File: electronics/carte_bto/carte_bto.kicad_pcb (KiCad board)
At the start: 2 copper layers, 160 x 100 mm, 192 parts, among them J1 DIN41612_02x32_AB, J2 Conn_01x01, J3 Conn_01x01, J4 Conn_01x01, J5 Conn_01x01, J6 Conn_01x01, Q1 MMBT2222A, Q10 MMBT2222A, Q11 MMBT2222A, Q12 MMBT2222A, Q13 MMBT2222A, Q14 MMBT2222A, Q15 MMBT2222A, Q16 MMBT2222A, Q17 MMBT2222A, Q18 MMBT2222A, Q2 MMBT2222A, Q3 MMBT2222A, Q4 MMBT2222A, Q5 MMBT2222A, Q6 MMBT2222A, Q7 MMBT2222A, Q8 MMBT2222A, Q9 MMBT2222A, U1 74AHC541, U2 LTC1859IG_PBF, U3 LT6654AIS6-2.5_TRPBF, U4 74AHC541, U5 L78L05_SOT89

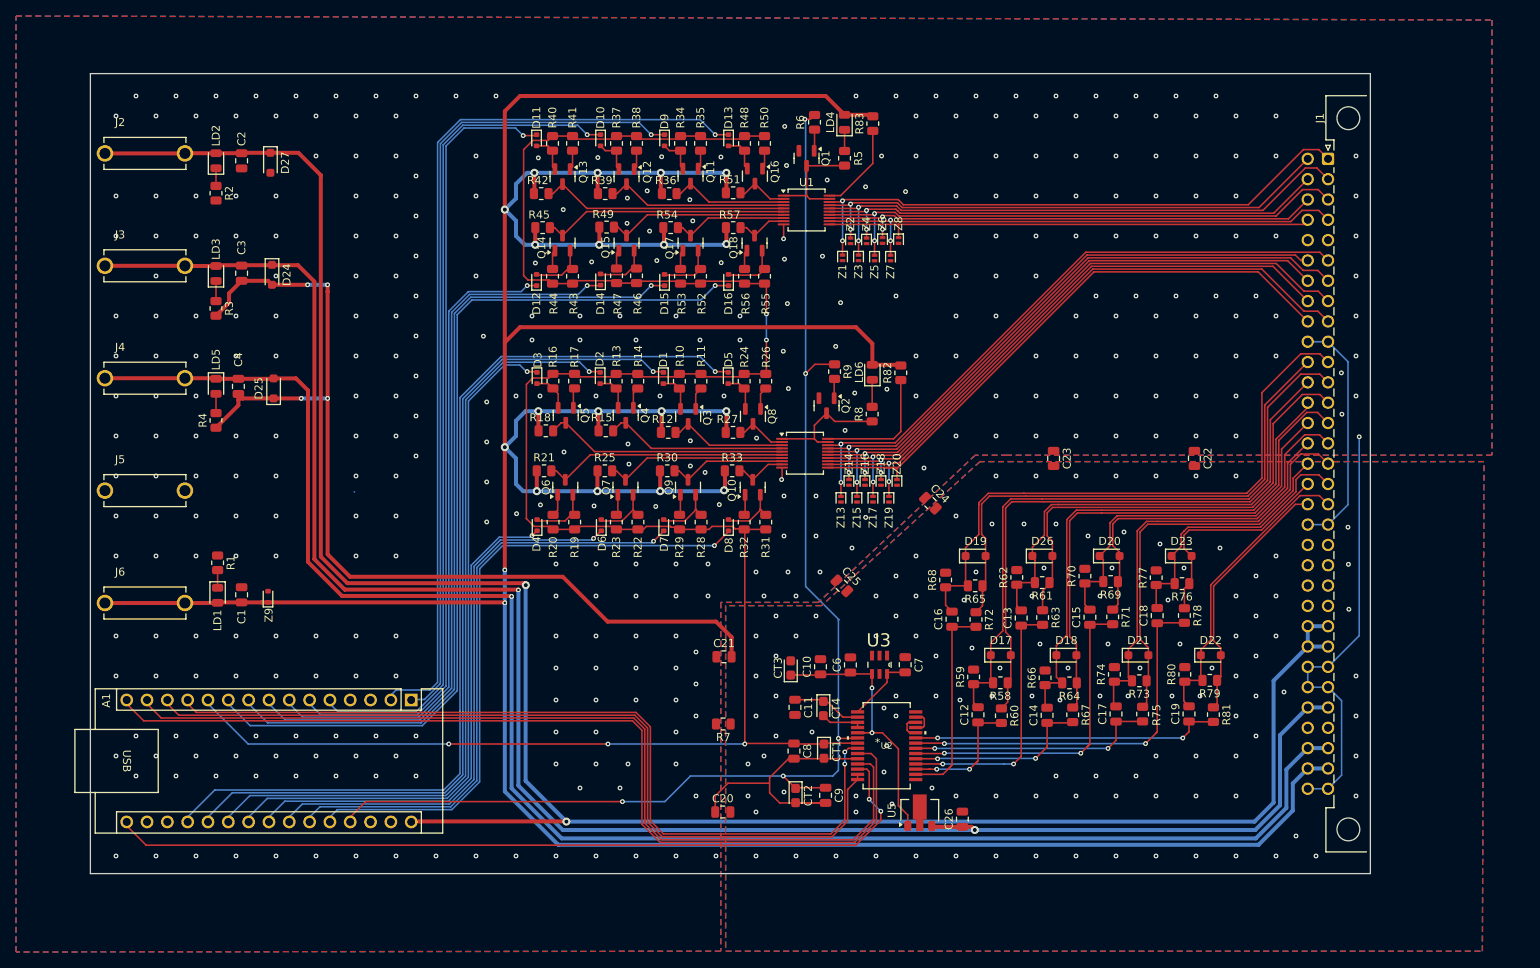
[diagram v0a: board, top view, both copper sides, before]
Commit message: BTO: Changed footprints to handsoldering verions, redid PCB routing
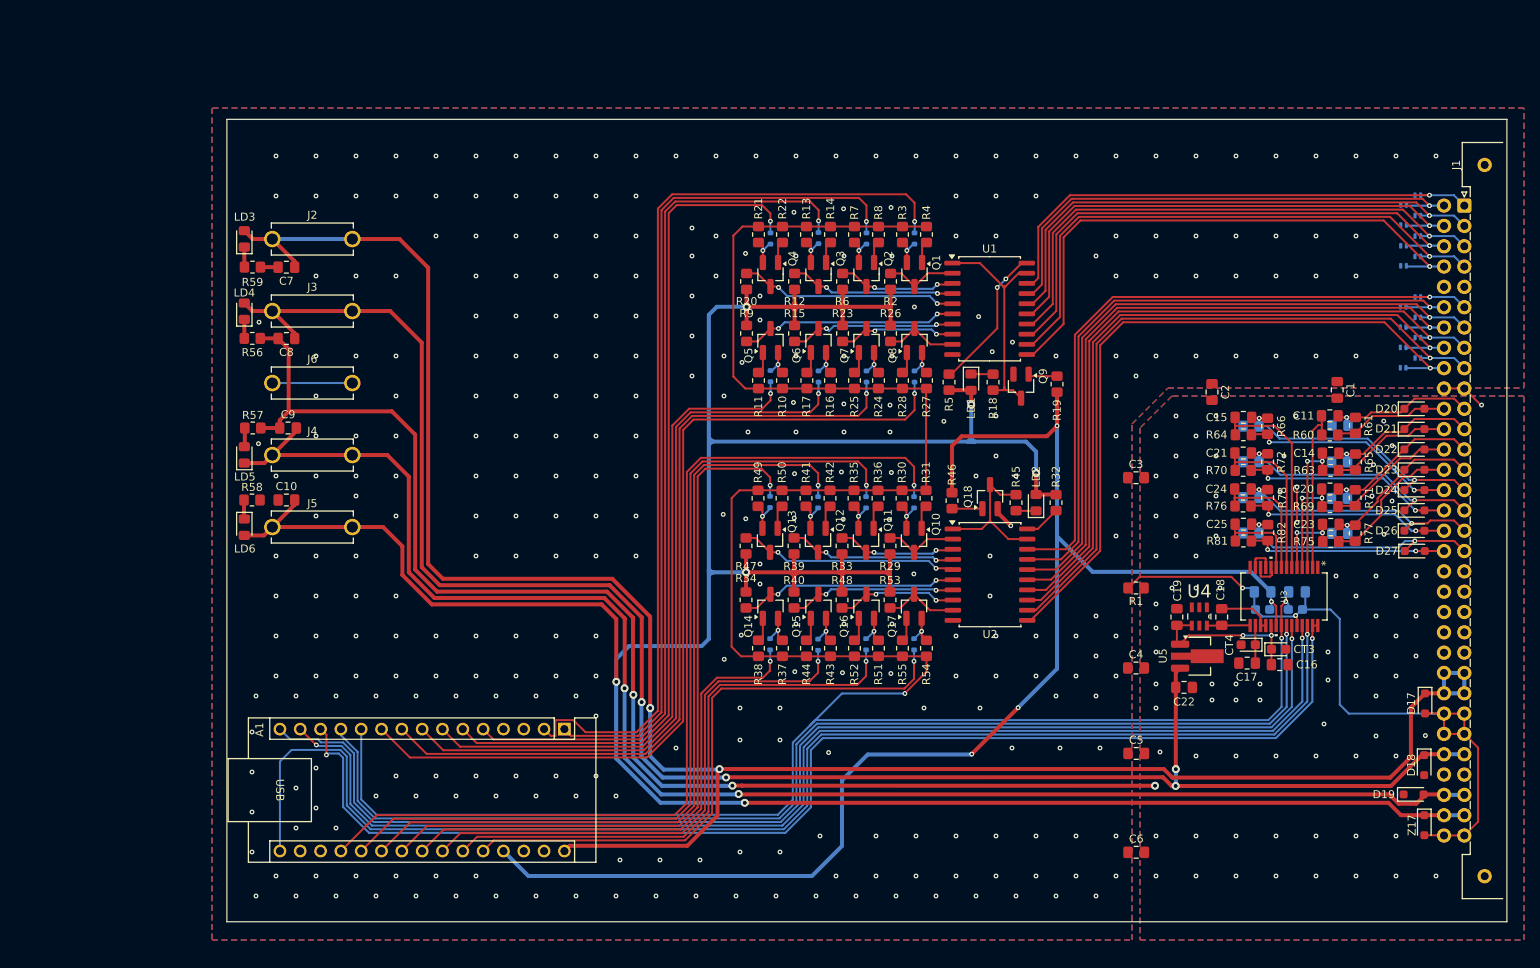
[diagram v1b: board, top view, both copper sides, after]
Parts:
- removed C26: 100nF, Capacitor_SMD:C_0805_2012Metric
- removed Z18, Z19, Z20: PESD5V0L1UL, Diode_SMD:D_SOD-882
- added C5: C_Small, Capacitor_SMD:C_0805_2012Metric_Pad1.18x1.45mm_HandSolder, F.Cu at (187.5, 124.7)
- added Z10: PESD5V0L1UL, PCM_Diode_SMD_Handsoldering_AKL:D_SOD-882_DFN1006-2_TVS, B.Cu at (220.9, 68.9)
- added Z11: PESD5V0L1UL, PCM_Diode_SMD_Handsoldering_AKL:D_SOD-882_DFN1006-2_TVS, B.Cu at (222.7, 70.2)
- added Z12: PESD5V0L1UL, PCM_Diode_SMD_Handsoldering_AKL:D_SOD-882_DFN1006-2_TVS, B.Cu at (220.9, 71.4)
- C1, C2, C3, C4: value 4.7µF -> C_Small; footprint Capacitor_SMD:C_0805_2012Metric -> Capacitor_SMD:C_0805_2012Metric_Pad1.18x1.45mm_HandSolder
- C10, C7, C8, C9: value 100nF -> 4.7µF; footprint Capacitor_SMD:C_0805_2012Metric -> Capacitor_SMD:C_0805_2012Metric_Pad1.18x1.45mm_HandSolder
- C11: value 100nF -> 1.5nF; footprint Capacitor_SMD:C_0805_2012Metric -> Capacitor_SMD:C_0805_2012Metric_Pad1.18x1.45mm_HandSolder
- C12, C13: value 1.5nF -> 100nF; footprint Capacitor_SMD:C_0805_2012Metric -> Capacitor_SMD:C_0805_2012Metric_Pad1.18x1.45mm_HandSolder; moved to B.Cu
- C14, C15: footprint Capacitor_SMD:C_0805_2012Metric -> Capacitor_SMD:C_0805_2012Metric_Pad1.18x1.45mm_HandSolder
- C16, C17, C18: value 1.5nF -> 100nF; footprint Capacitor_SMD:C_0805_2012Metric -> Capacitor_SMD:C_0805_2012Metric_Pad1.18x1.45mm_HandSolder
- C19: value 1.5nF -> 10µF; footprint Capacitor_SMD:C_0805_2012Metric -> Capacitor_SMD:C_0805_2012Metric_Pad1.18x1.45mm_HandSolder
- C20, C21, C23, C24, C25: value C_Small -> 1.5nF; footprint Capacitor_SMD:C_0805_2012Metric -> Capacitor_SMD:C_0805_2012Metric_Pad1.18x1.45mm_HandSolder
- C22: value C_Small -> 100nF; footprint Capacitor_SMD:C_0805_2012Metric -> Capacitor_SMD:C_0805_2012Metric_Pad1.18x1.45mm_HandSolder
- C6: value 10µF -> C_Small; footprint Capacitor_SMD:C_0805_2012Metric -> Capacitor_SMD:C_0805_2012Metric_Pad1.18x1.45mm_HandSolder
- CT1, CT2: moved to B.Cu
- D1, D10, D11, D12, D13, D14, D15, D16, D2, D3, D4, D5, D6, D7, D8, D9: footprint Diode_SMD:D_SOD-523 -> PCM_Diode_SMD_Handsoldering_AKL:D_SOD-523; moved to B.Cu
- D17: value SMAJ12CA -> SMAJ12A
- D18, D19: value SMAJ12CA -> SMAJ15A
- D20: value SMAJ12CA -> PESD12VL1BA
- D24, D25: value SMAJ15A -> SMAJ12CA
- D27: value SMAJ12A -> SMAJ12CA
- J1: footprint Connector_DIN:DIN41612_B_2x32_Male_Horizontal_THT -> connecteur_europe:DIN41612_B_2x32_Male_Horizontal_THT
- LD1, LD2: value LED_Small -> LED; footprint LED_SMD:LED_0805_2012Metric -> LED_SMD:LED_0805_2012Metric_Pad1.15x1.40mm_HandSolder
- LD3, LD5: footprint LED_SMD:LED_0805_2012Metric -> LED_SMD:LED_0805_2012Metric_Pad1.15x1.40mm_HandSolder
- LD4, LD6: value LED -> LED_Small; footprint LED_SMD:LED_0805_2012Metric -> LED_SMD:LED_0805_2012Metric_Pad1.15x1.40mm_HandSolder
- Q1, Q10, Q11, Q12, Q13, Q14, Q15, Q16, Q17, Q18, Q2, Q3, Q4, Q5, Q6, Q7, Q8, Q9: footprint Package_TO_SOT_SMD:SOT-23 -> Package_TO_SOT_SMD:SOT-23_Handsoldering
- R1, R5: value 3.3k -> 0; footprint Resistor_SMD:R_0805_2012Metric -> Resistor_SMD:R_0805_2012Metric_Pad1.20x1.40mm_HandSolder
- R10, R11, R12, R13, R16, R17, R21, R22, R23, R24, R27, R30, R33, R34, R37, R38, R39, R40, R43, R44, R48, R49, R50, R51, R54, R60, R61, R63, R65, R75, R81: footprint Resistor_SMD:R_0805_2012Metric -> Resistor_SMD:R_0805_2012Metric_Pad1.20x1.40mm_HandSolder
- R14, R20, R26, R29, R35, R41, R47, R53, R6, R9: value 22k -> 10k; footprint Resistor_SMD:R_0805_2012Metric -> Resistor_SMD:R_0805_2012Metric_Pad1.20x1.40mm_HandSolder
- R15, R19, R25, R28, R31, R36, R42, R46, R52, R55: value 10k -> 22k; footprint Resistor_SMD:R_0805_2012Metric -> Resistor_SMD:R_0805_2012Metric_Pad1.20x1.40mm_HandSolder
- R18, R45: value 10k -> 3.3k; footprint Resistor_SMD:R_0805_2012Metric -> Resistor_SMD:R_0805_2012Metric_Pad1.20x1.40mm_HandSolder
- R2, R3: value 5.1k -> 10k; footprint Resistor_SMD:R_0805_2012Metric -> Resistor_SMD:R_0805_2012Metric_Pad1.20x1.40mm_HandSolder
- R32: value 22k -> 0; footprint Resistor_SMD:R_0805_2012Metric -> Resistor_SMD:R_0805_2012Metric_Pad1.20x1.40mm_HandSolder
- R4: value 5.1k -> 22k; footprint Resistor_SMD:R_0805_2012Metric -> Resistor_SMD:R_0805_2012Metric_Pad1.20x1.40mm_HandSolder
- R56: value 22k -> 5.1k; footprint Resistor_SMD:R_0805_2012Metric -> Resistor_SMD:R_0805_2012Metric_Pad1.20x1.40mm_HandSolder
- R57: value 10k -> 5.1k; footprint Resistor_SMD:R_0805_2012Metric -> Resistor_SMD:R_0805_2012Metric_Pad1.20x1.40mm_HandSolder
- R58: value 1M -> 3.3k; footprint Resistor_SMD:R_0805_2012Metric -> Resistor_SMD:R_0805_2012Metric_Pad1.20x1.40mm_HandSolder
- R59: value 100 -> 5.1k; footprint Resistor_SMD:R_0805_2012Metric -> Resistor_SMD:R_0805_2012Metric_Pad1.20x1.40mm_HandSolder
- R62, R68, R74, R80: footprint Resistor_SMD:R_0805_2012Metric -> Resistor_SMD:R_0805_2012Metric_Pad1.20x1.40mm_HandSolder; moved to B.Cu
- R64, R69, R76: value 1M -> 10k; footprint Resistor_SMD:R_0805_2012Metric -> Resistor_SMD:R_0805_2012Metric_Pad1.20x1.40mm_HandSolder
- R66, R77: value 100 -> 1M; footprint Resistor_SMD:R_0805_2012Metric -> Resistor_SMD:R_0805_2012Metric_Pad1.20x1.40mm_HandSolder
- R67: value 10k -> 100; footprint Resistor_SMD:R_0805_2012Metric -> Resistor_SMD:R_0805_2012Metric_Pad1.20x1.40mm_HandSolder; moved to B.Cu
- R7: value 0 -> 10k; footprint Resistor_SMD:R_0805_2012Metric -> Resistor_SMD:R_0805_2012Metric_Pad1.20x1.40mm_HandSolder
- R70: value 100 -> 10k; footprint Resistor_SMD:R_0805_2012Metric -> Resistor_SMD:R_0805_2012Metric_Pad1.20x1.40mm_HandSolder
- R71, R72, R78: value 10k -> 1M; footprint Resistor_SMD:R_0805_2012Metric -> Resistor_SMD:R_0805_2012Metric_Pad1.20x1.40mm_HandSolder
- R73, R79: value 1M -> 100; footprint Resistor_SMD:R_0805_2012Metric -> Resistor_SMD:R_0805_2012Metric_Pad1.20x1.40mm_HandSolder; moved to B.Cu
- R8: value 3.3k -> 22k; footprint Resistor_SMD:R_0805_2012Metric -> Resistor_SMD:R_0805_2012Metric_Pad1.20x1.40mm_HandSolder
- R82: value 0 -> 1M; footprint Resistor_SMD:R_0805_2012Metric -> Resistor_SMD:R_0805_2012Metric_Pad1.20x1.40mm_HandSolder
- R83: value 0 -> 100; footprint Resistor_SMD:R_0805_2012Metric -> Resistor_SMD:R_0805_2012Metric_Pad1.20x1.40mm_HandSolder; moved to B.Cu
- U1: footprint Package_SO:TSSOP-20_4.4x5mm_P0.4mm -> Package_SO:SOIC-20W_7.5x12.8mm_P1.27mm
- U2: value LTC1859IG_PBF -> 74AHC541; footprint imported_components:SSOP-28_G -> Package_SO:SOIC-20W_7.5x12.8mm_P1.27mm
- U3: value LT6654AIS6-2.5_TRPBF -> LTC1859IG_PBF; footprint imported_components:SOT95P280X100-6N -> imported_components:SSOP-28_G
- U4: value 74AHC541 -> LT6654AIS6-2.5_TRPBF; footprint Package_SO:TSSOP-20_4.4x5mm_P0.4mm -> imported_components:SOT95P280X100-6N
- U5: footprint Package_TO_SOT_SMD:SOT-89-3 -> Package_TO_SOT_SMD:SOT-89-3_Handsoldering
- Z1, Z13, Z14, Z15, Z16, Z2, Z3, Z4, Z5, Z6, Z7, Z8: footprint Diode_SMD:D_SOD-882 -> PCM_Diode_SMD_Handsoldering_AKL:D_SOD-882_DFN1006-2_TVS; moved to B.Cu
- Z17: value PESD5V0L1UL -> PESD5V0L1UA; footprint Diode_SMD:D_SOD-882 -> Diode_SMD:D_SOD-323_HandSoldering
- Z9: footprint Diode_SMD:D_SOD-523 -> PCM_Diode_SMD_Handsoldering_AKL:D_SOD-882_DFN1006-2_TVS; moved to B.Cu
- moved D27 151.1 mm to (222.3, 99.4), turned to 0 degrees
- moved Z9 148.5 mm to (222.7, 67.6), turned to 180 degrees
- moved D24 145.3 mm to (222.3, 91.8), turned to 0 degrees
- moved D25 143.4 mm to (222.3, 94.3), turned to 0 degrees
- moved C1 139.3 mm to (212.7, 79.2), turned to -90 degrees
- moved C2 124.7 mm to (197.0, 79.5)
- moved C4 117.6 mm to (187.5, 114.0), turned to 0 degrees
- moved R1 114.8 mm to (187.5, 104.0), turned to 180 degrees
- moved C3 114.7 mm to (187.5, 90.2), turned to 0 degrees
- moved LD2 111.1 mm to (175.0, 93.3)
- moved R59 103.7 mm to (77.1, 63.9), turned to 0 degrees
- moved LD1 97.9 mm to (166.9, 78.3)
- moved R58 96.3 mm to (77.0, 93.0)
- moved C7 91.9 mm to (81.3, 63.9), turned to 180 degrees
- moved R4 91.8 mm to (161.3, 59.8), turned to -90 degrees
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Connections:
- net /d0 renamed /Bus donnée/OUT0
- net /d1 renamed /Bus donnée/OUT1
- net /d2 renamed /Bus donnée/OUT2
- net /d3 renamed /Bus donnée/OUT3
- net /d4 renamed /Bus donnée/OUT4
- net /d5 renamed /Bus donnée/OUT5
- net /d6 renamed /Bus donnée/OUT6
- net /d7 renamed /Bus donnée/OUT7
- A1 pad 12: /adc_busy -> /ADC 16 bits 8 voies/~{BUSY}
- A1 pad 13: /SPI.cs -> /ADC 16 bits 8 voies/SPI_CS
- A1 pad 14: /SPI.copi -> /ADC 16 bits 8 voies/SPI_COPI
- A1 pad 15: /SPI.cipo -> /ADC 16 bits 8 voies/SPI_CIPO
- A1 pad 16: /SPI.sck -> /ADC 16 bits 8 voies/SPI_SCK
- C1 pad 1: +5V -> GND2
- C1 pad 2: GND2 -> GND1
- C10 pad 1: +5VA -> +5V
- C10 pad 2: GND1 -> GND2
- C11 pad 1: Net-(U2-REFCOMP) -> /ADC 16 bits 8 voies/ch0
- C11 pad 2: GND1 -> /ADC 16 bits 8 voies/COM0_IN
- C12 pad 1: /Protections 8voies analogiques/CH1_OUT -> /ioref
- C12 pad 2: /acom1 -> GND2
- C13 pad 1: /Protections 8voies analogiques/CH2_OUT -> +5VARD
- C13 pad 2: /acom2 -> GND2
- C14 pad 1: /Protections 8voies analogiques/CH3_OUT -> /ADC 16 bits 8 voies/ch1
- C14 pad 2: /acom3 -> /ADC 16 bits 8 voies/COM1_IN
- C15 pad 1: /Protections 8voies analogiques/CH4_OUT -> /ADC 16 bits 8 voies/ch4
- C15 pad 2: /acom4 -> /ADC 16 bits 8 voies/COM4_IN
- C16 pad 1: /Protections 8voies analogiques/CH0_OUT -> +5VA
- C16 pad 2: /acom0 -> GND1
- C17 pad 1: /Protections 8voies analogiques/CH5_OUT -> Net-(U3-REFCOMP)
- C17 pad 2: /acom5 -> GND1
- C18 pad 1: /Protections 8voies analogiques/CH6_OUT -> Net-(U3-VREF)
- C18 pad 2: /acom6 -> GND1
- C19 pad 1: /Protections 8voies analogiques/CH7_OUT -> +5VA
- C19 pad 2: /acom7 -> GND1
- C2 pad 1: +12VP -> GND2
- C2 pad 2: GND2 -> GND1
- C20 pad 1: GND2 -> /ADC 16 bits 8 voies/ch2
- C20 pad 2: GND1 -> /ADC 16 bits 8 voies/COM2_IN
- C21 pad 1: GND2 -> /ADC 16 bits 8 voies/ch5
- C21 pad 2: GND1 -> /ADC 16 bits 8 voies/COM5_IN
- C22 pad 1: GND2 -> +15V
- C23 pad 1: GND2 -> /ADC 16 bits 8 voies/ch3
- C23 pad 2: GND1 -> /ADC 16 bits 8 voies/COM3_IN
- C24 pad 1: GND2 -> /ADC 16 bits 8 voies/ch6
- C24 pad 2: GND1 -> /ADC 16 bits 8 voies/COM6_IN
- C25 pad 1: GND2 -> /ADC 16 bits 8 voies/ch7
- C25 pad 2: GND1 -> /ADC 16 bits 8 voies/COM7_IN
- C3 pad 1: +15V -> GND2
- C4 pad 1: GND1 -> GND2
- C4 pad 2: -15V -> GND1
- C6 pad 1: +5VA -> GND2
- C7 pad 1: Net-(U2-VREF) -> +12VP
- C7 pad 2: GND1 -> GND2
- C8 pad 1: /ioref -> +15V
- C8 pad 2: GND2 -> GND1
- C9 pad 1: +5VARD -> GND1
- C9 pad 2: GND2 -> -15V
- CT4 pad 1: Net-(U2-REFCOMP) -> Net-(U3-REFCOMP)
- D1 pad 1: /addr1 -> /data0
- D10 pad 1: /data2 -> /addr1
- D11 pad 1: /data3 -> /addr2
- D12 pad 1: /data4 -> /addr3
- D13 pad 1: /data0 -> /addr4
- D14 pad 1: /data5 -> /addr5
- D15 pad 1: /data6 -> /addr6
- D16 pad 1: /data7 -> /addr7
- D17 pad 1: /acom1 -> +12VP
- D17 pad 2: /ach1 -> GND2
- D18 pad 1: /acom3 -> +15V
- D18 pad 2: /ach3 -> GND1
- D19 pad 1: /acom0 -> GND1
- D19 pad 2: /ach0 -> -15V
- D2 pad 1: /addr2 -> /data1
- D20 pad 1: /acom4 -> /ADC 16 bits 8 voies/COM0_IN
- D20 pad 2: /ach4 -> /ADC 16 bits 8 voies/CH0_IN
- D21 pad 1: /acom5 -> /ADC 16 bits 8 voies/COM1_IN
- D21 pad 2: /ach5 -> /ADC 16 bits 8 voies/CH1_IN
- D22 pad 1: /acom7 -> /ADC 16 bits 8 voies/COM2_IN
- D22 pad 2: /ach7 -> /ADC 16 bits 8 voies/CH2_IN
- D23 pad 1: /acom6 -> /ADC 16 bits 8 voies/COM3_IN
- D23 pad 2: /ach6 -> /ADC 16 bits 8 voies/CH3_IN
- D24 pad 1: +15V -> /ADC 16 bits 8 voies/COM4_IN
- D24 pad 2: GND1 -> /ADC 16 bits 8 voies/CH4_IN
- D25 pad 1: GND1 -> /ADC 16 bits 8 voies/COM5_IN
- D25 pad 2: -15V -> /ADC 16 bits 8 voies/CH5_IN
- D26 pad 1: /acom2 -> /ADC 16 bits 8 voies/COM6_IN
- D26 pad 2: /ach2 -> /ADC 16 bits 8 voies/CH6_IN
- D27 pad 1: +12VP -> /ADC 16 bits 8 voies/COM7_IN
- D27 pad 2: GND2 -> /ADC 16 bits 8 voies/CH7_IN
- D3 pad 1: /addr3 -> /data2
- D4 pad 1: /addr4 -> /data3
- D5 pad 1: /addr0 -> /data4
- D6 pad 1: /addr5 -> /data5
- D7 pad 1: /addr6 -> /data6
- D8 pad 1: /addr7 -> /data7
- D9 pad 1: /data1 -> /addr0
- J1 pad a11: /acom0 -> /ADC 16 bits 8 voies/COM0_IN
- J1 pad a12: /acom1 -> /ADC 16 bits 8 voies/COM1_IN
- J1 pad a13: /acom2 -> /ADC 16 bits 8 voies/COM2_IN
- J1 pad a14: /acom3 -> /ADC 16 bits 8 voies/COM3_IN
- J1 pad a15: /acom4 -> /ADC 16 bits 8 voies/COM4_IN
- J1 pad a16: /acom5 -> /ADC 16 bits 8 voies/COM5_IN
- J1 pad a17: /acom6 -> /ADC 16 bits 8 voies/COM6_IN
- J1 pad a18: /acom7 -> /ADC 16 bits 8 voies/COM7_IN
- J1 pad a6: /a0 -> /Bus d’adresse/OUT0
- J1 pad a7: /a2 -> /Bus d’adresse/OUT2
- J1 pad a8: /a4 -> /Bus d’adresse/OUT4
- J1 pad a9: /a6 -> /Bus d’adresse/OUT6
- J1 pad b11: /ach0 -> /ADC 16 bits 8 voies/CH0_IN
- J1 pad b12: /ach1 -> /ADC 16 bits 8 voies/CH1_IN
- J1 pad b13: /ach2 -> /ADC 16 bits 8 voies/CH2_IN
- J1 pad b14: /ach3 -> /ADC 16 bits 8 voies/CH3_IN
- J1 pad b15: /ach4 -> /ADC 16 bits 8 voies/CH4_IN
- J1 pad b16: /ach5 -> /ADC 16 bits 8 voies/CH5_IN
- J1 pad b17: /ach6 -> /ADC 16 bits 8 voies/CH6_IN
- J1 pad b18: /ach7 -> /ADC 16 bits 8 voies/CH7_IN
- J1 pad b6: /a1 -> /Bus d’adresse/OUT1
- J1 pad b7: /a3 -> /Bus d’adresse/OUT3
- J1 pad b8: /a5 -> /Bus d’adresse/OUT5
- J1 pad b9: /a7 -> /Bus d’adresse/OUT7
- J5 pad 1_1: GND2 -> +5V
- J5 pad 1_2: GND2 -> +5V
- J6 pad 1_1: +5V -> GND2
- J6 pad 1_2: +5V -> GND2
- LD2 pad 2: +12VP -> +5V
- LD3 pad 2: +15V -> +12VP
- LD4 pad 2: +5V -> +15V
- Q1 pad 2: GND2 -> Net-(D1-A)
- Q1 pad 3: Net-(Q1-C) -> /Bus donnée/bit0
- Q10 pad 2: Net-(D8-A) -> Net-(D9-A)
- Q10 pad 3: /Adaptateur 3v3 - 5v 8voies (1)/OUT7 -> /Bus d’adresse/bit0
- Q11 pad 2: Net-(D9-A) -> Net-(D10-A)
- Q11 pad 3: /Adaptateur 3v3 - 5v 8voies (2)/OUT1 -> /Bus d’adresse/bit1
- Q12 pad 2: Net-(D10-A) -> Net-(D11-A)
- Q12 pad 3: /Adaptateur 3v3 - 5v 8voies (2)/OUT2 -> /Bus d’adresse/bit2
- Q13 pad 2: Net-(D11-A) -> Net-(D12-A)
- Q13 pad 3: /Adaptateur 3v3 - 5v 8voies (2)/OUT3 -> /Bus d’adresse/bit3
- Q14 pad 2: Net-(D12-A) -> Net-(D13-A)
- Q14 pad 3: /Adaptateur 3v3 - 5v 8voies (2)/OUT4 -> /Bus d’adresse/bit4
- Q15 pad 3: /Adaptateur 3v3 - 5v 8voies (2)/OUT5 -> /Bus d’adresse/bit5
- Q16 pad 2: Net-(D13-A) -> Net-(D15-A)
- Q16 pad 3: /Adaptateur 3v3 - 5v 8voies (2)/OUT0 -> /Bus d’adresse/bit6
- Q17 pad 2: Net-(D15-A) -> Net-(D16-A)
- Q17 pad 3: /Adaptateur 3v3 - 5v 8voies (2)/OUT6 -> /Bus d’adresse/bit7
- Q18 pad 2: Net-(D16-A) -> GND2
- Q18 pad 3: /Adaptateur 3v3 - 5v 8voies (2)/OUT7 -> Net-(Q18-C)
- Q2 pad 2: GND2 -> Net-(D2-A)
- Q2 pad 3: Net-(Q2-C) -> /Bus donnée/bit1
- Q3 pad 2: Net-(D1-A) -> Net-(D3-A)
- Q3 pad 3: /Adaptateur 3v3 - 5v 8voies (1)/OUT1 -> /Bus donnée/bit2
- Q4 pad 2: Net-(D2-A) -> Net-(D4-A)
- Q4 pad 3: /Adaptateur 3v3 - 5v 8voies (1)/OUT2 -> /Bus donnée/bit3
- Q5 pad 2: Net-(D3-A) -> Net-(D5-A)
- Q5 pad 3: /Adaptateur 3v3 - 5v 8voies (1)/OUT3 -> /Bus donnée/bit4
- Q6 pad 2: Net-(D4-A) -> Net-(D6-A)
- Q6 pad 3: /Adaptateur 3v3 - 5v 8voies (1)/OUT4 -> /Bus donnée/bit5
- Q7 pad 2: Net-(D6-A) -> Net-(D7-A)
- Q7 pad 3: /Adaptateur 3v3 - 5v 8voies (1)/OUT5 -> /Bus donnée/bit6
- Q8 pad 2: Net-(D5-A) -> Net-(D8-A)
- Q8 pad 3: /Adaptateur 3v3 - 5v 8voies (1)/OUT0 -> /Bus donnée/bit7
- Q9 pad 2: Net-(D7-A) -> GND2
- Q9 pad 3: /Adaptateur 3v3 - 5v 8voies (1)/OUT6 -> Net-(Q9-C)
- R1 pad 1: GND2 -> GND1
- R1 pad 2: Net-(LD1-K) -> GND2
- R10 pad 2: Net-(D1-A) -> Net-(D5-A)
- R11 pad 2: Net-(Q3-B) -> Net-(Q5-B)
- R12 pad 2: /Adaptateur 3v3 - 5v 8voies (1)/OUT1 -> /Bus donnée/bit2
- R13 pad 2: Net-(D2-A) -> Net-(D3-A)
- R14 pad 2: Net-(Q4-B) -> Net-(Q3-B)
- R15 pad 2: /Adaptateur 3v3 - 5v 8voies (1)/OUT2 -> /Bus donnée/bit5
- R16 pad 2: Net-(D3-A) -> Net-(D6-A)
- R17 pad 2: Net-(Q5-B) -> Net-(Q6-B)
- R18 pad 1: +5V -> Net-(Q9-C)
- R18 pad 2: /Adaptateur 3v3 - 5v 8voies (1)/OUT3 -> Net-(LD1-K)
- R19 pad 1: /ioref -> +5VARD
- R19 pad 2: Net-(D4-A) -> Net-(Q9-B)
- R2 pad 1: Net-(LD2-K) -> +5V
- R2 pad 2: GND2 -> /Bus donnée/bit0
- R20 pad 1: /ioref -> +5V
- R20 pad 2: Net-(Q6-B) -> /Bus donnée/bit3
- R21 pad 1: +5V -> /ioref
- R21 pad 2: /Adaptateur 3v3 - 5v 8voies (1)/OUT4 -> Net-(D4-A)
- R22 pad 2: Net-(D6-A) -> Net-(Q4-B)
- R23 pad 1: /ioref -> +5V
- R23 pad 2: Net-(Q7-B) -> /Bus donnée/bit6
- R24 pad 2: Net-(D5-A) -> Net-(D7-A)
- R25 pad 1: +5V -> /ioref
- R25 pad 2: /Adaptateur 3v3 - 5v 8voies (1)/OUT5 -> Net-(Q7-B)
- R26 pad 1: /ioref -> +5V
- R26 pad 2: Net-(Q8-B) -> /Bus donnée/bit7
- R27 pad 1: +5V -> /ioref
- R27 pad 2: /Adaptateur 3v3 - 5v 8voies (1)/OUT0 -> Net-(D8-A)
- R28 pad 2: Net-(D7-A) -> Net-(Q8-B)
- R29 pad 1: /ioref -> +5V
- R29 pad 2: Net-(Q9-B) -> /Bus d’adresse/bit0
- R3 pad 1: Net-(LD3-K) -> /ioref
- R3 pad 2: GND1 -> Net-(D1-A)
- R30 pad 1: +5V -> /ioref
- R30 pad 2: /Adaptateur 3v3 - 5v 8voies (1)/OUT6 -> Net-(D9-A)
- R31 pad 2: Net-(D8-A) -> Net-(Q10-B)
- R32 pad 1: /ioref -> Net-(U2-VCC)
- R32 pad 2: Net-(Q10-B) -> +5V
- R33 pad 2: /Adaptateur 3v3 - 5v 8voies (1)/OUT7 -> /Bus d’adresse/bit1
- R34 pad 1: /ioref -> +5V
- R34 pad 2: Net-(D9-A) -> /Bus d’adresse/bit4
- R35 pad 2: Net-(Q11-B) -> Net-(D10-A)
- R36 pad 1: +5V -> /ioref
- R36 pad 2: /Adaptateur 3v3 - 5v 8voies (2)/OUT1 -> Net-(Q11-B)
- R37 pad 2: Net-(D10-A) -> Net-(D13-A)
- R38 pad 2: Net-(Q12-B) -> Net-(Q14-B)
- R39 pad 2: /Adaptateur 3v3 - 5v 8voies (2)/OUT2 -> /Bus d’adresse/bit2
- R4 pad 1: GND1 -> /ioref
- R4 pad 2: Net-(LD5-A) -> Net-(Q1-B)
- R40 pad 1: /ioref -> +5V
- R40 pad 2: Net-(D11-A) -> /Bus d’adresse/bit5
- R41 pad 2: Net-(Q13-B) -> Net-(D11-A)
- R42 pad 1: +5V -> /ioref
- R42 pad 2: /Adaptateur 3v3 - 5v 8voies (2)/OUT3 -> Net-(Q12-B)
- R43 pad 2: Net-(D12-A) -> Net-(D14-A)
- R44 pad 2: Net-(Q14-B) -> Net-(Q15-B)
- R45 pad 1: +5V -> Net-(Q18-C)
- R45 pad 2: /Adaptateur 3v3 - 5v 8voies (2)/OUT4 -> Net-(LD2-K)
- R46 pad 1: /ioref -> +5VARD
- R46 pad 2: Net-(D14-A) -> Net-(Q18-B)
- R47 pad 1: /ioref -> +5V
- R47 pad 2: Net-(Q15-B) -> /Bus d’adresse/bit3
- R48 pad 1: /ioref -> +5V
- R48 pad 2: Net-(D13-A) -> /Bus d’adresse/bit6
- R49 pad 1: +5V -> /ioref
- R49 pad 2: /Adaptateur 3v3 - 5v 8voies (2)/OUT5 -> Net-(D12-A)
- R5 pad 1: Net-(Q1-C) -> Net-(U1-VCC)
- R5 pad 2: Net-(LD4-K) -> +5V
- R50 pad 2: Net-(Q16-B) -> Net-(Q13-B)
- R51 pad 1: +5V -> /ioref
- R51 pad 2: /Adaptateur 3v3 - 5v 8voies (2)/OUT0 -> Net-(D15-A)
- R52 pad 2: Net-(D15-A) -> Net-(Q16-B)
- R53 pad 1: /ioref -> +5V
- R53 pad 2: Net-(Q17-B) -> /Bus d’adresse/bit7
- R54 pad 1: +5V -> /ioref
- R54 pad 2: /Adaptateur 3v3 - 5v 8voies (2)/OUT6 -> Net-(D16-A)
- R55 pad 2: Net-(D16-A) -> Net-(Q17-B)
- R56 pad 1: /ioref -> Net-(LD4-K)
- R56 pad 2: Net-(Q18-B) -> GND1
- R57 pad 1: +5V -> GND1
- R57 pad 2: /Adaptateur 3v3 - 5v 8voies (2)/OUT7 -> Net-(LD5-A)
- R58 pad 1: /ach1 -> GND2
- R58 pad 2: /acom1 -> Net-(LD6-K)
- R59 pad 1: /acom1 -> Net-(LD3-K)
- R59 pad 2: GND1 -> GND2
- R6 pad 1: +5VARD -> +5V
- R6 pad 2: Net-(Q1-B) -> /Bus donnée/bit1
- R60 pad 1: /ach1 -> /ADC 16 bits 8 voies/CH0_IN
- R60 pad 2: /Protections 8voies analogiques/CH1_OUT -> /ADC 16 bits 8 voies/ch0
- R61 pad 1: /ach2 -> /ADC 16 bits 8 voies/CH0_IN
- R61 pad 2: /acom2 -> /ADC 16 bits 8 voies/COM0_IN
- R62 pad 1: /acom2 -> /ADC 16 bits 8 voies/COM0_IN
- R63 pad 1: /ach2 -> /ADC 16 bits 8 voies/CH1_IN
- R63 pad 2: /Protections 8voies analogiques/CH2_OUT -> /ADC 16 bits 8 voies/ch1
- R64 pad 1: /ach3 -> /ADC 16 bits 8 voies/CH4_IN
- R64 pad 2: /acom3 -> /ADC 16 bits 8 voies/ch4
- R65 pad 1: /ach0 -> /ADC 16 bits 8 voies/CH1_IN
- R65 pad 2: /acom0 -> /ADC 16 bits 8 voies/COM1_IN
- R66 pad 1: /acom3 -> /ADC 16 bits 8 voies/CH4_IN
- R66 pad 2: GND1 -> /ADC 16 bits 8 voies/COM4_IN
- R67 pad 1: /ach3 -> /ADC 16 bits 8 voies/COM1_IN
- R67 pad 2: /Protections 8voies analogiques/CH3_OUT -> GND1
- R68 pad 1: /acom0 -> /ADC 16 bits 8 voies/COM4_IN
- R69 pad 1: /ach4 -> /ADC 16 bits 8 voies/CH2_IN
- R69 pad 2: /acom4 -> /ADC 16 bits 8 voies/ch2
- R7 pad 1: GND1 -> /ioref
- R7 pad 2: GND2 -> Net-(D2-A)
- R70 pad 1: /acom4 -> /ADC 16 bits 8 voies/CH5_IN
- R70 pad 2: GND1 -> /ADC 16 bits 8 voies/ch5
- R71 pad 1: /ach4 -> /ADC 16 bits 8 voies/CH2_IN
- R71 pad 2: /Protections 8voies analogiques/CH4_OUT -> /ADC 16 bits 8 voies/COM2_IN
- R72 pad 1: /ach0 -> /ADC 16 bits 8 voies/CH5_IN
- R72 pad 2: /Protections 8voies analogiques/CH0_OUT -> /ADC 16 bits 8 voies/COM5_IN
- R73 pad 1: /ach5 -> /ADC 16 bits 8 voies/COM2_IN
- R73 pad 2: /acom5 -> GND1
- R74 pad 1: /acom5 -> /ADC 16 bits 8 voies/COM5_IN
- R75 pad 1: /ach5 -> /ADC 16 bits 8 voies/CH3_IN
- R75 pad 2: /Protections 8voies analogiques/CH5_OUT -> /ADC 16 bits 8 voies/ch3
- R76 pad 1: /ach6 -> /ADC 16 bits 8 voies/CH6_IN
- R76 pad 2: /acom6 -> /ADC 16 bits 8 voies/ch6
- R77 pad 1: /acom6 -> /ADC 16 bits 8 voies/CH3_IN
- R77 pad 2: GND1 -> /ADC 16 bits 8 voies/COM3_IN
- R78 pad 1: /ach6 -> /ADC 16 bits 8 voies/CH6_IN
- R78 pad 2: /Protections 8voies analogiques/CH6_OUT -> /ADC 16 bits 8 voies/COM6_IN
- R79 pad 1: /ach7 -> /ADC 16 bits 8 voies/COM3_IN
- R79 pad 2: /acom7 -> GND1
- R8 pad 1: Net-(Q2-C) -> /ioref
- R8 pad 2: Net-(LD6-K) -> Net-(Q2-B)
- R80 pad 1: /acom7 -> /ADC 16 bits 8 voies/COM6_IN
- R81 pad 1: /ach7 -> /ADC 16 bits 8 voies/CH7_IN
- R81 pad 2: /Protections 8voies analogiques/CH7_OUT -> /ADC 16 bits 8 voies/ch7
- R82 pad 1: Net-(U4-VCC) -> /ADC 16 bits 8 voies/CH7_IN
- R82 pad 2: +5V -> /ADC 16 bits 8 voies/COM7_IN
- R83 pad 1: Net-(U1-VCC) -> /ADC 16 bits 8 voies/COM7_IN
- R83 pad 2: +5V -> GND1
- R9 pad 1: +5VARD -> +5V
- R9 pad 2: Net-(Q2-B) -> /Bus donnée/bit4
- U1 pad 1: Net-(Q1-C) -> Net-(Q9-C)
- U1 pad 19: Net-(Q1-C) -> Net-(Q9-C)
- U1 pad 2: /Adaptateur 3v3 - 5v 8voies (2)/OUT0 -> /Bus donnée/bit0
- U1 pad 3: /Adaptateur 3v3 - 5v 8voies (2)/OUT1 -> /Bus donnée/bit1
- U1 pad 4: /Adaptateur 3v3 - 5v 8voies (2)/OUT2 -> /Bus donnée/bit2
- U1 pad 5: /Adaptateur 3v3 - 5v 8voies (2)/OUT3 -> /Bus donnée/bit3
- U1 pad 6: /Adaptateur 3v3 - 5v 8voies (2)/OUT4 -> /Bus donnée/bit4
- U1 pad 7: /Adaptateur 3v3 - 5v 8voies (2)/OUT5 -> /Bus donnée/bit5
- U1 pad 8: /Adaptateur 3v3 - 5v 8voies (2)/OUT6 -> /Bus donnée/bit6
- U1 pad 9: /Adaptateur 3v3 - 5v 8voies (2)/OUT7 -> /Bus donnée/bit7
- U2 pad 1: GND1 -> Net-(Q18-C)
- U2 pad 10: Net-(U2-ADC+) -> GND2
- U2 pad 11: Net-(U2-ADC-) -> /Bus d’adresse/OUT7
- U2 pad 12: Net-(U2-ADC+) -> /Bus d’adresse/OUT6
- U2 pad 13: Net-(U2-ADC-) -> /Bus d’adresse/OUT5
- U2 pad 14: GND1 -> /Bus d’adresse/OUT4
- U2 pad 15: Net-(U2-VREF) -> /Bus d’adresse/OUT3
- U2 pad 16: Net-(U2-REFCOMP) -> /Bus d’adresse/OUT2
- U2 pad 17: GND1 -> /Bus d’adresse/OUT1
- U2 pad 18: GND1 -> /Bus d’adresse/OUT0
- U2 pad 19: +5VA -> Net-(Q18-C)
- U2 pad 2: /Protections 8voies analogiques/CH0_OUT -> /Bus d’adresse/bit0
- U2 pad 20: +5VARD -> Net-(U2-VCC)
- U2 pad 3: /Protections 8voies analogiques/CH1_OUT -> /Bus d’adresse/bit1
- U2 pad 4: /Protections 8voies analogiques/CH2_OUT -> /Bus d’adresse/bit2
- U2 pad 5: /Protections 8voies analogiques/CH3_OUT -> /Bus d’adresse/bit3
- U2 pad 6: /Protections 8voies analogiques/CH4_OUT -> /Bus d’adresse/bit4
- U2 pad 7: /Protections 8voies analogiques/CH5_OUT -> /Bus d’adresse/bit5
- U2 pad 8: /Protections 8voies analogiques/CH6_OUT -> /Bus d’adresse/bit6
- U2 pad 9: /Protections 8voies analogiques/CH7_OUT -> /Bus d’adresse/bit7
- U3 pad 2: GND1 -> /ADC 16 bits 8 voies/ch0
- U3 pad 3: unconnected-(U3-DNC-Pad3) -> /ADC 16 bits 8 voies/ch1
- U3 pad 4: +5VA -> /ADC 16 bits 8 voies/ch2
- U3 pad 5: unconnected-(U3-DNC_2-Pad5) -> /ADC 16 bits 8 voies/ch3
- U3 pad 6: Net-(U2-VREF) -> /ADC 16 bits 8 voies/ch4
- U4 pad 1: Net-(Q2-C) -> GND1
- U4 pad 2: /Adaptateur 3v3 - 5v 8voies (1)/OUT0 -> GND1
- U4 pad 3: /Adaptateur 3v3 - 5v 8voies (1)/OUT1 -> unconnected-(U4-DNC-Pad3)
- U4 pad 4: /Adaptateur 3v3 - 5v 8voies (1)/OUT2 -> +5VA
- U4 pad 5: /Adaptateur 3v3 - 5v 8voies (1)/OUT3 -> unconnected-(U4-DNC_2-Pad5)
- U4 pad 6: /Adaptateur 3v3 - 5v 8voies (1)/OUT4 -> Net-(U3-VREF)
- Z13 pad 1: /a0 -> /Bus d’adresse/OUT4
- Z14 pad 1: /a1 -> /Bus d’adresse/OUT5
- Z15 pad 1: /a2 -> /Bus d’adresse/OUT6
- Z16 pad 1: /a3 -> /Bus d’adresse/OUT7
- Z17 pad 1: /a4 -> +5V
- Z9 pad 1: +5V -> /Bus d’adresse/OUT0
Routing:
- net /ADC 16 bits 8 voies/SPI_SCK: track 0.00 -> 168.2 mm, vias 0 -> 1
- net /ADC 16 bits 8 voies/SPI_CS: track 0.00 -> 155.7 mm, vias 0 -> 2
- net /ADC 16 bits 8 voies/SPI_CIPO: track 0.00 -> 155.2 mm, vias 0 -> 1
- net /ADC 16 bits 8 voies/SPI_COPI: track 0.00 -> 154.0 mm, vias 0 -> 2
- net /ADC 16 bits 8 voies/~{BUSY}: track 0.00 -> 146.7 mm, vias 0 -> 1
- net /SPI.cipo: track 119.7 -> 0.00 mm
- net /SPI.copi: track 115.0 -> 0.00 mm
- net +5V: track 511.5 -> 400.2 mm, vias 20 -> 6
- net /adc_busy: track 107.2 -> 0.00 mm, vias 2 -> 0
- net /SPI.cs: track 106.4 -> 0.00 mm
- net /SPI.sck: track 105.2 -> 0.00 mm, vias 2 -> 0
- net /Bus d’adresse/OUT6: track 0.00 -> 88.4 mm, vias 0 -> 1
- net /Bus d’adresse/OUT7: track 0.00 -> 87.9 mm, vias 0 -> 1
- net /Bus d’adresse/OUT4: track 0.00 -> 87.1 mm, vias 0 -> 1
- net /Bus d’adresse/OUT5: track 0.00 -> 86.5 mm, vias 0 -> 1
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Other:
- board size 160 x 100 mm -> 160 x 100.3 mm
